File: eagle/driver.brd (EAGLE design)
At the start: 101.6 x 76.2 mm, 89 parts, among them IC1 XMEGA128A1, IC10 ST95P08M, IC11 ST95P08M, IC12 ST95P08M, IC13 ST95P08M, IC14 ST95P08M, IC15 ST95P08M, IC16 74AHC1G02DBV, IC17 74AHC1G02DBV, IC18 74AHC1G125DBV, IC19 74AHC1G125DBV, IC2 74AC16244, IC20 ST95P08M, IC21 ST95P08M, IC22 ST95P08M, IC23 ST95P08M, IC24 ST95P08M, IC25 ST95P08M, IC3 74AC16244, IC4 74AC16244, IC5 74AC16244, IC6 74AC16374, IC7 74AC16374, IC8 74AC16374, IC9 74AC16374

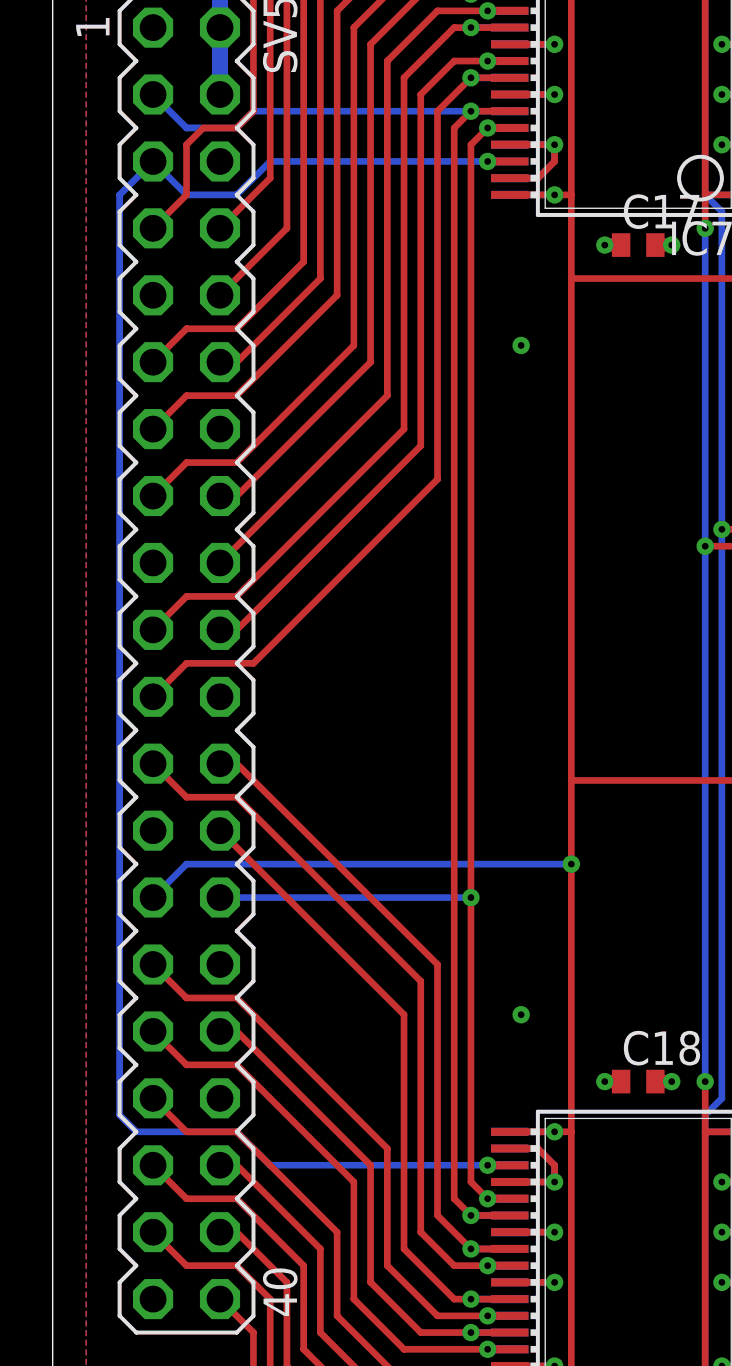
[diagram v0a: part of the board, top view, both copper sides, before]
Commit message: finalizing board layout
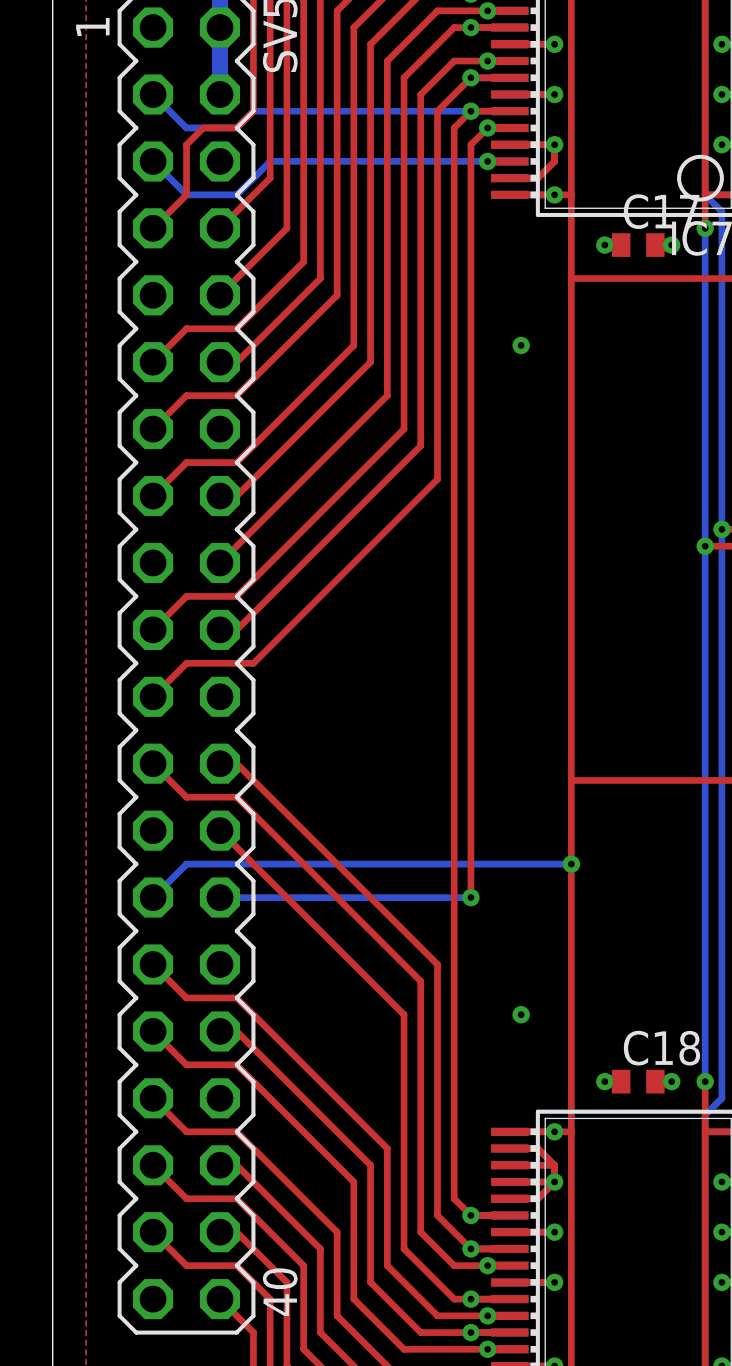
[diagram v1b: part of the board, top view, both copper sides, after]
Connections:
- net GND: now also IC8.27, IC8.29, IC9.44, IC9.46
- net N$92: no longer IC8.27, IC9.46
- net N$93: no longer IC8.29, IC9.44
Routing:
- net N$92: track 68.6 -> 15.4 mm, vias 2 -> 1
- net N$93: track 54.0 -> 40.7 mm, vias 3 -> 2
- net GND: track 180.2 -> 187.5 mm
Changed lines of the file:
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@@
 <wire x1="17.3482" y1="11.43" x2="19.05" y2="11.43" width="0.254" layer="16"/>
 <wire x1="17.3482" y1="14.605" x2="19.05" y2="14.605" width="0.254" layer="16"/>
-<wire x1="17.3482" y1="18.415" x2="19.05" y2="18.415" width="0.254" layer="16"/>
 <wire x1="27.1018" y1="18.415" x2="25.4" y2="18.415" width="0.254" layer="16"/>
 <wire x1="27.1018" y1="14.605" x2="25.4" y2="14.605" width="0.254" layer="16"/>
@@
 <via x="67.31" y="73.025" extent="1-16" drill="0.254"/>
 <via x="78.74" y="73.025" extent="1-16" drill="0.254"/>
+<contactref element="IC8" pad="27"/>
+<contactref element="IC9" pad="46"/>
+<contactref element="IC8" pad="29"/>
+<contactref element="IC9" pad="44"/>
+<wire x1="17.3482" y1="17.78" x2="18.415" y2="17.78" width="0.254" layer="1"/>
+<wire x1="18.415" y1="17.78" x2="19.05" y2="18.415" width="0.254" layer="1"/>
+<wire x1="17.3482" y1="19.05" x2="19.05" y2="19.05" width="0.254" layer="1"/>
+<wire x1="17.3482" y1="19.05" x2="19.05" y2="19.05" width="0.254" layer="16"/>
+<wire x1="17.3482" y1="18.415" x2="19.05" y2="18.415" width="0.254" layer="16"/>
+<wire x1="17.3482" y1="17.78" x2="18.415" y2="17.78" width="0.254" layer="16"/>
+<wire x1="18.415" y1="17.78" x2="19.05" y2="18.415" width="0.254" layer="16"/>
 </signal>
 <signal name="VCC">
@@
 <via x="16.51" y="57.15" extent="1-16" drill="0.254"/>
 <wire x1="17.3482" y1="57.15" x2="16.51" y2="57.15" width="0.254" layer="1"/>
-<contactref element="IC8" pad="27"/>
-<contactref element="IC9" pad="46"/>
-<wire x1="3.81" y1="57.15" x2="2.54" y2="55.88" width="0.254" layer="16"/>
-<wire x1="2.54" y1="55.88" x2="2.54" y2="20.955" width="0.254" layer="16"/>
-<wire x1="2.54" y1="20.955" x2="3.175" y2="20.32" width="0.254" layer="16"/>
-<wire x1="3.175" y1="20.32" x2="6.985" y2="20.32" width="0.254" layer="16"/>
-<wire x1="6.985" y1="20.32" x2="8.255" y2="19.05" width="0.254" layer="16"/>
-<wire x1="8.255" y1="19.05" x2="16.51" y2="19.05" width="0.254" layer="16"/>
-<wire x1="16.51" y1="19.05" x2="17.3482" y2="19.05" width="0.254" layer="16"/>
 <wire x1="3.81" y1="57.15" x2="5.08" y2="55.88" width="0.254" layer="16"/>
 <wire x1="5.08" y1="55.88" x2="6.985" y2="55.88" width="0.254" layer="16"/>
 <wire x1="6.985" y1="55.88" x2="8.255" y2="57.15" width="0.254" layer="16"/>
 <wire x1="8.255" y1="57.15" x2="16.51" y2="57.15" width="0.254" layer="16"/>
-<wire x1="17.3482" y1="19.05" x2="16.51" y2="19.05" width="0.254" layer="1"/>
-<via x="16.51" y="19.05" extent="1-16" drill="0.254"/>
 </signal>
 <signal name="N$93">
@@
 <via x="16.51" y="58.42" extent="1-16" drill="0.254"/>
 <wire x1="17.3482" y1="58.42" x2="16.51" y2="58.42" width="0.254" layer="16"/>
-<contactref element="IC8" pad="29"/>
-<contactref element="IC9" pad="44"/>
-<wire x1="15.875" y1="29.21" x2="15.875" y2="18.415" width="0.254" layer="1"/>
-<wire x1="15.875" y1="18.415" x2="16.51" y2="17.78" width="0.254" layer="1"/>
-<wire x1="16.51" y1="17.78" x2="17.3482" y2="17.78" width="0.254" layer="1"/>
-<via x="16.51" y="17.78" extent="1-16" drill="0.254"/>
-<wire x1="17.3482" y1="17.78" x2="16.51" y2="17.78" width="0.254" layer="16"/>
 </signal>
 <signal name="N$35">
